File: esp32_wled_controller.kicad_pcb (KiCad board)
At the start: 4 copper layers, 95 x 95 mm, 83 parts, among them J1 USB_C_Receptacle_USB2.0_16P, J2 Screw_Terminal_01x03, J3 Screw_Terminal_01x03, J4 Screw_Terminal_01x03, J5 Screw_Terminal_01x03, J6 Screw_Terminal_01x02, J7 Screw_Terminal_01x02, K1 SRD-05VDC-SL-C, K2 SRD-05VDC-SL-C, K3 SRD-05VDC-SL-C, K4 SRD-05VDC-SL-C, Q1 SS8050, Q2 SS8050, Q3 BC547A, Q4 BC547A, Q5 BC547A, Q6 BC547A, U1 USBLC6-2P6, U10 ESP32-S2-WROOM, U2 AMS1117-3.3, U3 CP2104, U5 PC817, U6 PC817, U7 PC817, U8 PC817, U9 SN74AHCT125PWR

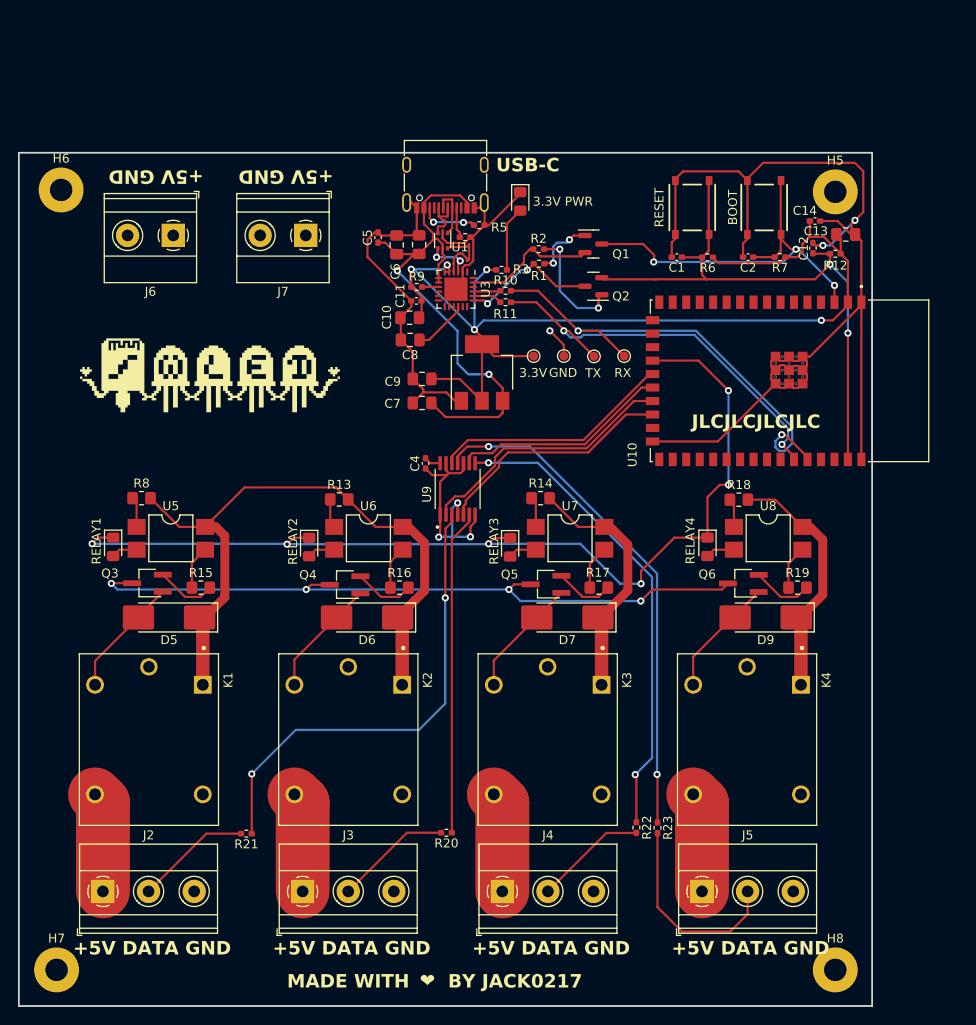
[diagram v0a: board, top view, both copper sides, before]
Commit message: board rev 1.2, cleanup
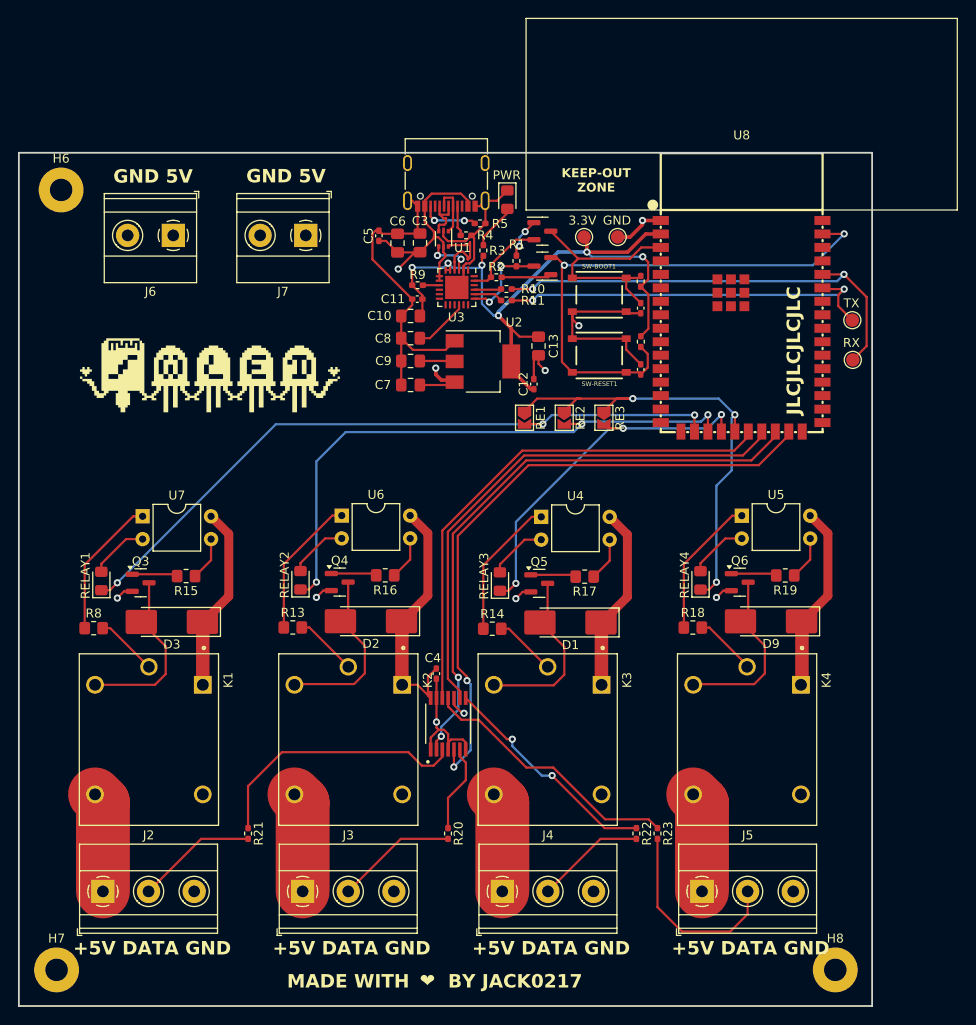
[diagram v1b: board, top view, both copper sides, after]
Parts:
- removed 3.3V1, RX2, TX2: TestPoint, TestPoint:TestPoint_Pad_D1.0mm
- removed BOOT, RESET: SW_SPST, lib:TS-1187A-B-A-B
- removed C14: 100nF, Capacitor_SMD:C_0402_1005Metric_Pad0.74x0.62mm_HandSolder
- removed D5, D6, D7: 1N4007, Diode_SMD:D_MELF_Handsoldering
- removed H5: MountingHole_Pad, MountingHole:MountingHole_2.5mm_Pad
- removed R12: 1K, Resistor_SMD:R_0402_1005Metric_Pad0.72x0.64mm_HandSolder
- removed U10: ESP32-S2-WROOM, lib:XCVR_ESP32-S2-WROOM
- added 3V3: TestPoint, TestPoint:TestPoint_Pad_D1.5mm, F.Cu at (84.2, 30.3)
- added D1: C7420350, Diode_SMD:D_MELF_Handsoldering, F.Cu at (82.7, 73.2)
- added D2: C7420350, Diode_SMD:D_MELF_Handsoldering, F.Cu at (60.4, 73.1)
- added D3: C7420350, Diode_SMD:D_MELF_Handsoldering, F.Cu at (38.3, 73.1)
- added RE1: SolderJumper_2_Bridged, Jumper:SolderJumper-2_P1.3mm_Open_TrianglePad1.0x1.5mm, F.Cu at (77.5, 50.4)
- added RE2: SolderJumper_2_Bridged, Jumper:SolderJumper-2_P1.3mm_Open_TrianglePad1.0x1.5mm, F.Cu at (82.0, 50.4)
- added RE3: SolderJumper_2_Bridged, Jumper:SolderJumper-2_P1.3mm_Open_TrianglePad1.0x1.5mm, F.Cu at (86.4, 50.4)
- added REF**: OSHW-Logo_11.4x12mm_SilkScreen, Symbol:OSHW-Logo_11.4x12mm_SilkScreen, B.Cu at (108.1, 34.4)
- added RX1: TestPoint, TestPoint:TestPoint_Pad_D1.5mm, F.Cu at (114.1, 44.0)
- added SW-BOOT1: SW_SPST, lib:TS-1187A-B-A-B, F.Cu at (85.9, 36.7)
- added SW-RESET1: SW_SPST, lib:TS-1187A-B-A-B, F.Cu at (85.9, 43.5)
- added TX1: TestPoint, TestPoint:TestPoint_Pad_D1.5mm, F.Cu at (114.0, 39.5)
- added U4: EL817, Package_DIP:DIP-4_W7.62mm, F.Cu at (79.4, 61.4)
- D9: value 1N4007 -> C7420350
- GND1: footprint TestPoint:TestPoint_Pad_D1.0mm -> TestPoint:TestPoint_Pad_D1.5mm
- Q3, Q4, Q5, Q6: value BC547A -> SS8050; footprint Package_TO_SOT_SMD:TSOT-23_HandSoldering -> Package_TO_SOT_SMD:SOT-23
- U5, U6, U7: value PC817 -> EL817; footprint Package_DIP:SMDIP-4_W7.62mm -> Package_DIP:DIP-4_W7.62mm
- U8: value PC817 -> ESP32-S2-WROOM-1-N4(4MB); footprint Package_DIP:SMDIP-4_W7.62mm -> lib:WIFI-SMD_ESP32-S2-WROVER-I
- moved U5 63.6 mm to (101.7, 61.3)
- moved U7 47.7 mm to (35.0, 61.4)
- moved C13 36.4 mm to (79.1, 42.4), turned to -90 degrees
- moved C12 34.6 mm to (78.6, 46.7)
- moved U9 26.2 mm to (69.0, 84.5)
- moved U8 23.8 mm to (101.7, 40.2)
- moved C4 23.4 mm to (67.7, 78.9)
- moved R7 15.7 mm to (90.5, 35.2), turned to 90 degrees
- moved R14 15.5 mm to (74.0, 73.9)
- moved R8 15.4 mm to (29.6, 73.8)
- moved R13 15.2 mm to (51.7, 73.8)
- moved R18 15.1 mm to (96.3, 73.8)
- moved GND1 14.5 mm to (87.9, 30.3), turned to 0 degrees
- moved C2 13.2 mm to (90.5, 38.2), turned to -90 degrees
- moved C1 13.1 mm to (90.5, 45.0), turned to 90 degrees
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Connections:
- C12 pad 1: /EN -> +3.3V
- C4 pad 1: Net-(U9-GND) -> GND
- C4 pad 2: Net-(U9-VCC) -> +5V
- K1 pad A2: Net-(D5-A) -> Net-(D3-A)
- K2 pad A2: Net-(D6-A) -> Net-(D2-A)
- K3 pad A2: Net-(D7-A) -> Net-(D1-A)
- Q3 pad 1: Net-(D5-A) -> Net-(Q3-B)
- Q3 pad 2: Net-(Q3-B) -> GND
- Q3 pad 3: GND -> Net-(D3-A)
- Q4 pad 1: Net-(D6-A) -> Net-(Q4-B)
- Q4 pad 2: Net-(Q4-B) -> GND
- Q4 pad 3: GND -> Net-(D2-A)
- Q5 pad 1: Net-(D7-A) -> Net-(Q5-B)
- Q5 pad 2: Net-(Q5-B) -> GND
- Q5 pad 3: GND -> Net-(D1-A)
- Q6 pad 1: Net-(D9-A) -> Net-(Q6-B)
- Q6 pad 2: Net-(Q6-B) -> GND
- Q6 pad 3: GND -> Net-(D9-A)
- RELAY1 pad 1: /IO17_RELAYS -> /RELAY1
- RELAY2 pad 1: /IO17_RELAYS -> /RELAY2
- RELAY3 pad 1: /IO17_RELAYS -> /RELAY3
- RELAY4 pad 1: /IO17_RELAYS -> /RELAY4
- U5 pad 1: Net-(R8-Pad1) -> Net-(R18-Pad1)
- U5 pad 2: Net-(RELAY1-A) -> Net-(RELAY4-A)
- U5 pad 3: Net-(R15-Pad1) -> Net-(R19-Pad1)
- U7 pad 1: Net-(R14-Pad1) -> Net-(R8-Pad1)
- U7 pad 2: Net-(RELAY3-A) -> Net-(RELAY1-A)
- U7 pad 3: Net-(R17-Pad1) -> Net-(R15-Pad1)
- U8 pad 1: Net-(R18-Pad1) -> GND
- U8 pad 2: Net-(RELAY4-A) -> +3.3V
- U8 pad 3: Net-(R19-Pad1) -> /IO0
- U8 pad 4: +5V -> unconnected-(U8-IO1-Pad4)
- U9 pad 1: Net-(U9-GND) -> GND
- U9 pad 10: Net-(U9-GND) -> GND
- U9 pad 13: Net-(U9-GND) -> GND
- U9 pad 14: Net-(U9-VCC) -> +5V
- U9 pad 4: Net-(U9-GND) -> GND
- U9 pad 7: Net-(U9-GND) -> GND
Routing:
- net GND: track 270.2 -> 114.3 mm, vias 7 -> 9
- net /IO17_RELAYS: track 109.2 -> 0.00 mm, vias 6 -> 0
- net /RELAY1: track 0.00 -> 78.0 mm, vias 0 -> 3
- net /RELAY2: track 0.00 -> 65.1 mm, vias 0 -> 3
- net /RELAY4: track 0.00 -> 54.4 mm, vias 0 -> 3
- net /STRIP2: track 26.8 -> 70.9 mm, vias 0 -> 2
- net /RELAY3: track 0.00 -> 41.0 mm, vias 0 -> 3
- net +3.3V: track 120.9 -> 81.5 mm, vias 5 -> 6
- net /STRIP1: track 29.4 -> 66.2 mm, vias 0 -> 2
- net +5V: track 188.6 -> 153.1 mm
- net /STRIP3: track 24.3 -> 59.0 mm
- net /STRIP4: track 26.9 -> 57.6 mm
- net Net-(U9-3Y): track 53.1 -> 25.5 mm
- net Net-(U9-4Y): track 57.0 -> 29.9 mm, vias 2 -> 0
- net Net-(U9-GND): track 26.4 -> 0.00 mm, vias 3 -> 0
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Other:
- board text added: "GND 5V"
- board text added: "KEEP-OUT ZONE"
- board text added: "PWR"
- board text added: "website: jack0217.dev github: @fellettigiacomo license: CERN-OHL-S"
- board text removed: "+5V GND"
- board text removed: "3.3V PWR"
- board text removed: "USB-C"
